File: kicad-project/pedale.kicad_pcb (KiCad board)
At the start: 2 copper layers, 121.5 x 81.5 mm, 45 parts, among them IC1 TLV76150DCYR, IC2 TLV76150DCYR, IC3 TLV76150DCYR, IC4 TLV76150DCYR, IC5 TLV76150DCYR

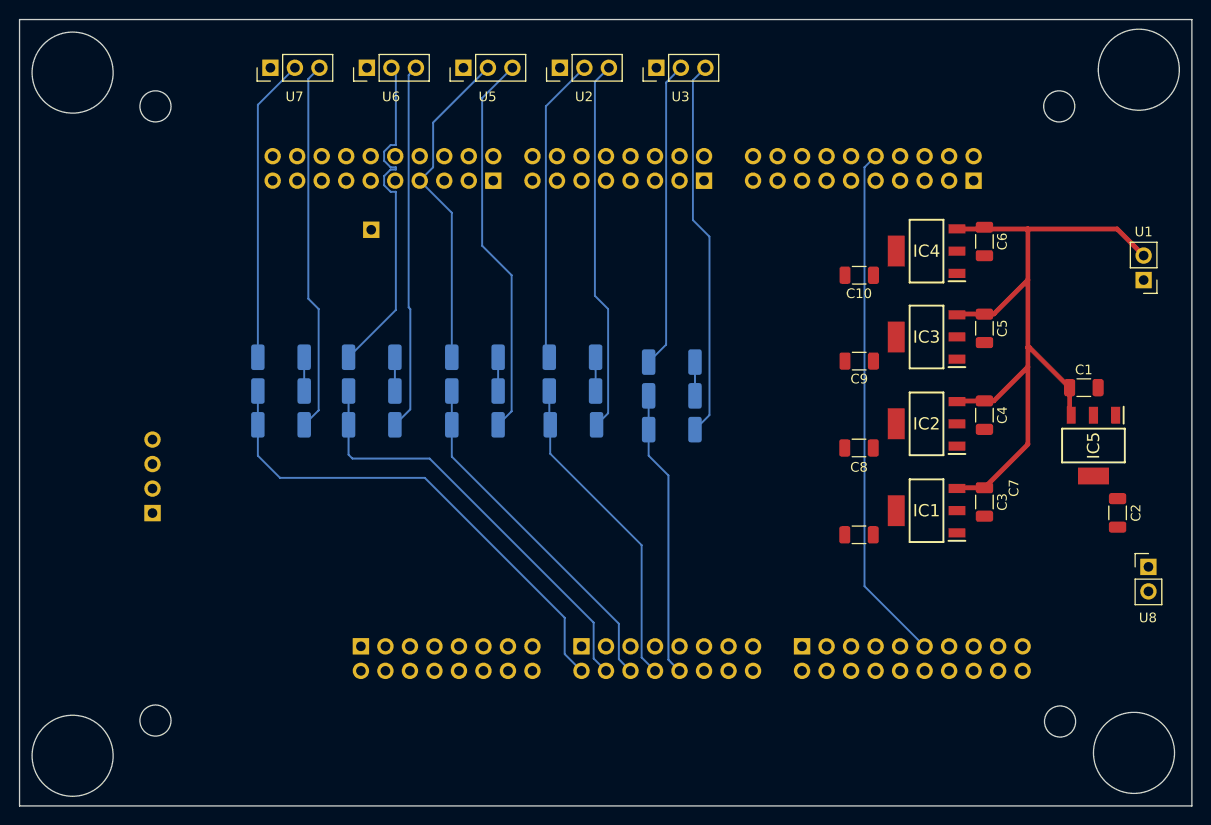
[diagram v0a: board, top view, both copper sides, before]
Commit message: modificari
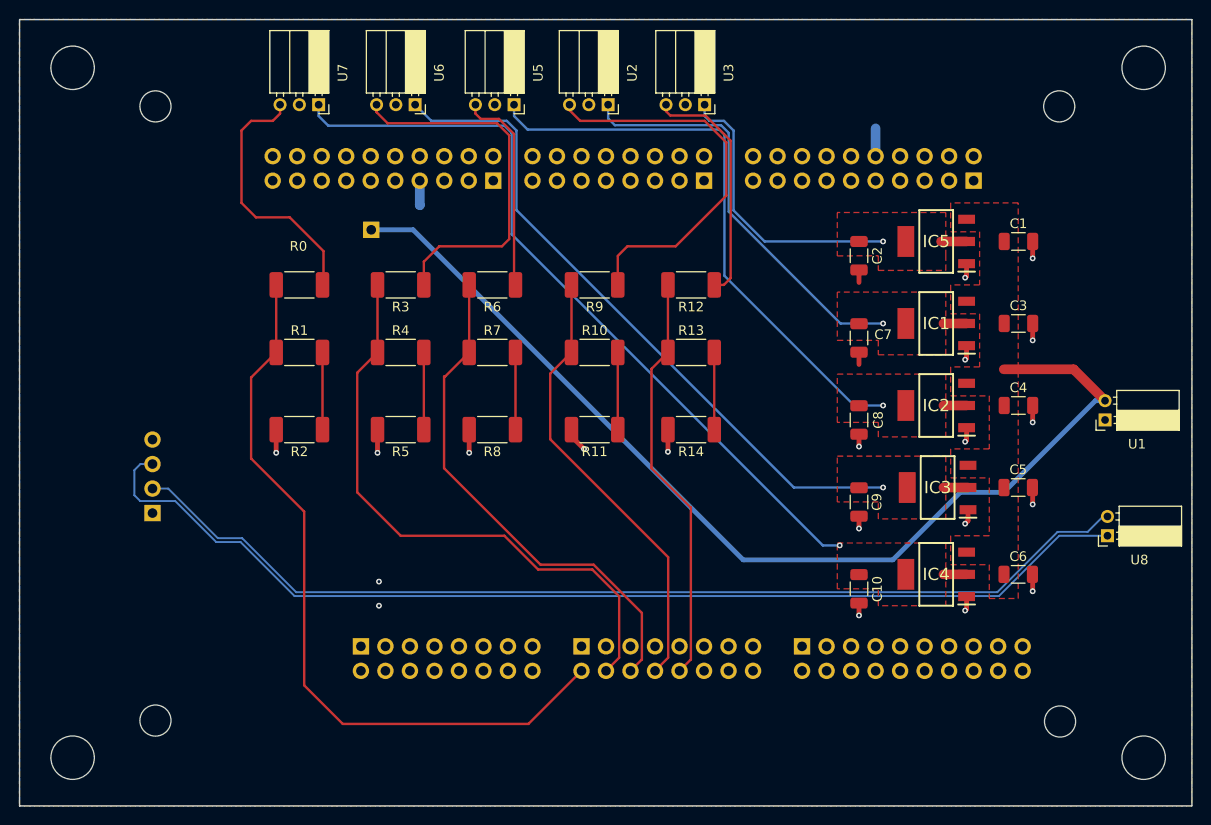
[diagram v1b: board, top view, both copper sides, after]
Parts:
- R0, R1, R10, R11, R12, R13, R14, R2, R3, R4, R5, R6, R7, R8, R9: moved to F.Cu
- U1, U8: footprint Connector_PinHeader_2.54mm:PinHeader_1x02_P2.54mm_Vertical -> Connector_PinSocket_2.00mm:PinSocket_1x02_P2.00mm_Horizontal
- U2, U3, U5, U6, U7: footprint Connector_PinHeader_2.54mm:PinHeader_1x03_P2.54mm_Vertical -> Connector_PinSocket_2.00mm:PinSocket_1x03_P2.00mm_Horizontal
- moved C2 37.8 mm to (104.5, 45.0)
- moved C6 34.7 mm to (121.0, 78.0), turned to 0 degrees
- moved IC4 33.5 mm to (112.5, 78.0)
- moved C10 32.5 mm to (104.5, 79.5), turned to -90 degrees
- moved IC5 26.7 mm to (112.5, 43.5), turned to 180 degrees
- moved C7 20.4 mm to (104.5, 53.5), turned to -90 degrees
- moved IC1 19.4 mm to (112.5, 52.0)
- moved C3 18.8 mm to (121.0, 52.0), turned to 0 degrees
- moved C5 16.9 mm to (121.0, 69.0), turned to 0 degrees
- moved C1 16.6 mm to (121.0, 43.5)
- moved IC3 15.6 mm to (112.7, 69.0)
- moved R12 15.1 mm to (87.1, 48.0)
- moved U1 15.0 mm to (130.0, 62.0)
- moved R3 14.8 mm to (57.0, 48.0)
- moved R9 14.7 mm to (77.1, 48.0)
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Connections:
- net Net-(IC1-IN) renamed 12V
- net Net-(IC1-OUT_1) renamed /5V_2
- net Net-(IC2-OUT_1) renamed /5V_3
- net Net-(IC3-OUT_1) renamed /5V_4
- net Net-(IC4-OUT_1) renamed /5V_5
- net Net-(IC5-OUT_1) renamed /5V_1
- net Net-(U4-CANH) renamed /CAN_P
- net Net-(U4-CANL) renamed /CAN_N
- J13 pad 12: unconnected-(J13-GND-Pad12) -> GND
- J13 pad 14: unconnected-(J13-GND-Pad14) -> GND
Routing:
- net GND: track 218.9 -> 40.3 mm, vias 0 -> 20
- net /CAN_P: track 0.00 -> 112.8 mm
- net /CAN_N: track 0.00 -> 106.7 mm
- net /5V_5: track 0.00 -> 82.2 mm, vias 0 -> 1
- net /5V_4: track 0.00 -> 72.3 mm, vias 0 -> 1
- net /5V_3: track 0.00 -> 62.8 mm, vias 0 -> 1
- net /5V_2: track 0.00 -> 45.9 mm, vias 0 -> 1
- net /5V_1: track 0.00 -> 32.6 mm, vias 0 -> 1
- net 12V: track 78.7 -> 108.9 mm
- net Net-(J14-ptd1): track 51.7 -> 77.5 mm
- net Net-(U5-A0): track 40.1 -> 21.5 mm
- net Net-(J14-ptd0): track 44.7 -> 62.3 mm
- net Net-(J14-pta13): track 36.7 -> 53.3 mm
- net Net-(U3-A0): track 39.4 -> 24.9 mm
- net Net-(J14-pta9): track 29.8 -> 42.9 mm
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- added copper zone on F.Cu, net /5V_1
- added copper zone on F.Cu, net /5V_2
- added copper zone on F.Cu, net /5V_3
- added copper zone on F.Cu, net /5V_4
- added copper zone on F.Cu, net /5V_5
- added copper zone on F.Cu, net 12V
- added copper zone on B.Cu, net GND
- added copper zone on F.Cu, net GND
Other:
- outline, holes or cut-outs redrawn
